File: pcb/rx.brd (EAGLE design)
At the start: 20 x 40 mm, 8 parts, among them IC1 REG1117, IC2 STM32F042K6, J1 USB_A_PTH_MALE

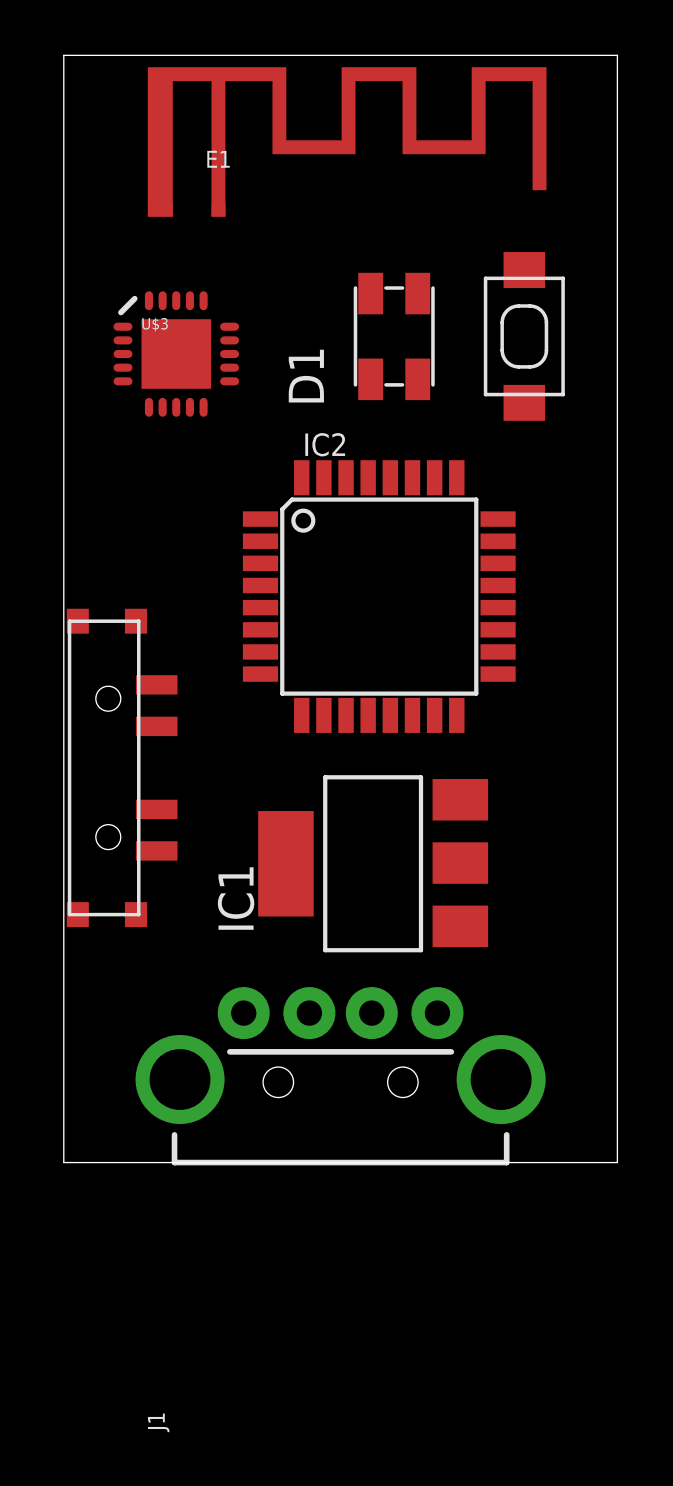
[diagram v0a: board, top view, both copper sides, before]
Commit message: cleanup
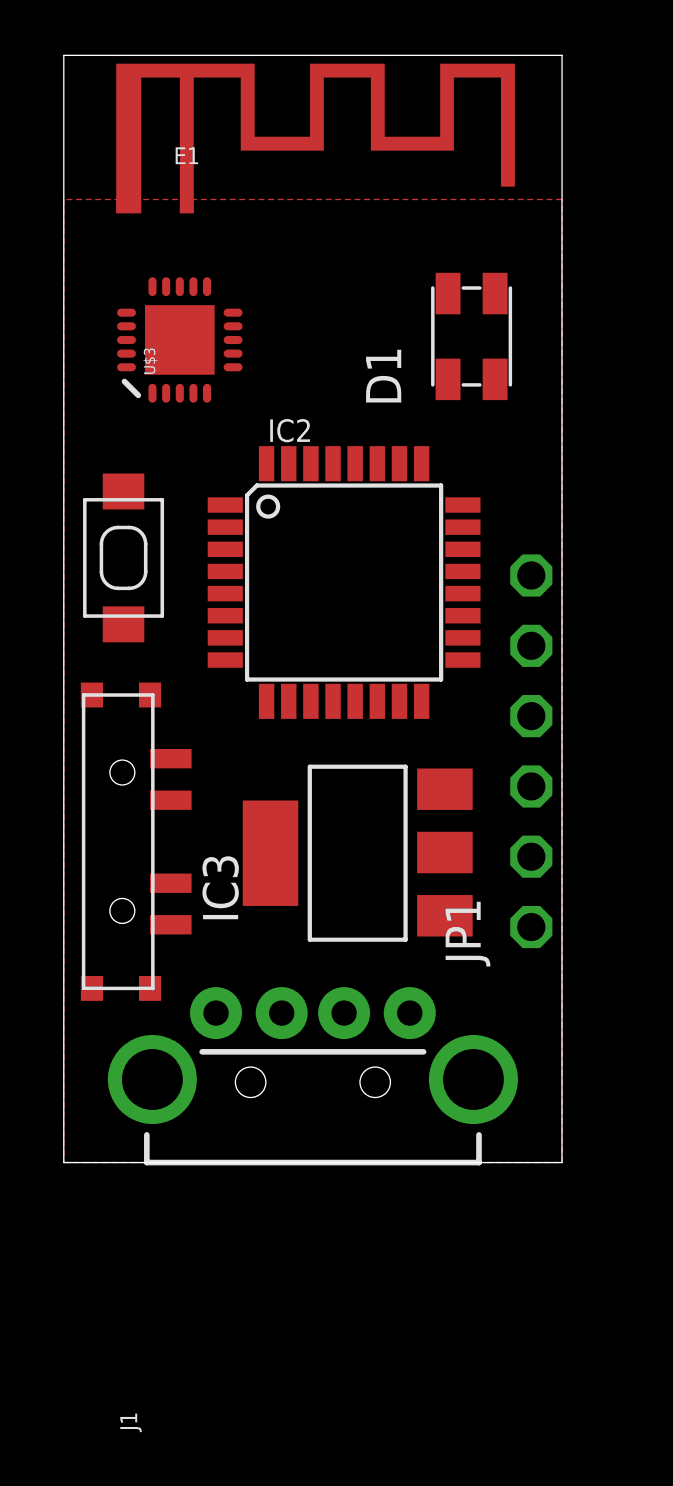
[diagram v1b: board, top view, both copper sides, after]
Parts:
- removed IC1: REG1117, usbclogger:SOT223
- added IC3: REG1117, clock:SOT223
- added JP1: (no value), adafruit:1X06-CLEAN
- moved S1 16.5 mm to (2.16, 21.8)
- moved D1 2.79 mm to (14.7, 29.8)
- moved U$1 2.71 mm to (1.02, 16.9)
- moved IC2 1.37 mm to (10.1, 21.0)
- moved E1 1.15 mm to (4.45, 34.8)
- moved J1 1.00 mm to (9.00, 3.00)
- moved U$3 0.52 mm to (4.19, 29.7), turned to 90 degrees
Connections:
- net GND: now also IC3.1; no longer IC1.1
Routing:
- added copper zone on layer 1, net GND
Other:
- board size 20 x 40 mm -> 18 x 40 mm
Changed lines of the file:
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@@
 <board>
 <plain>
-<wire x1="0" y1="0" x2="20" y2="0" width="0" layer="20"/>
-<wire x1="20" y1="0" x2="20" y2="40" width="0" layer="20"/>
-<wire x1="20" y1="40" x2="0" y2="40" width="0" layer="20"/>
+<wire x1="0" y1="0" x2="18" y2="0" width="0" layer="20"/>
+<wire x1="18" y1="0" x2="18" y2="40" width="0" layer="20"/>
+<wire x1="18" y1="40" x2="0" y2="40" width="0" layer="20"/>
 <wire x1="0" y1="40" x2="0" y2="0" width="0" layer="20"/>
 </plain>
@@
 </autorouter>
 <elements>
-<element name="U$3" library="nRF24L01-Chip-v13" package="QFN20_ALT1" value="NRF24L01ALT1" x="4.064" y="29.21"/>
-<element name="J1" library="SparkFun-Connectors" package="USB-A-H" value="USB_A_PTH_MALE" x="10" y="3" rot="R90">
-<attribute name="PROD_ID" value="CONN-08367" x="10" y="3" size="1.778" layer="27" rot="R90" display="off"/>
-<attribute name="SF_ID" value="PRT-00437" x="10" y="3" size="1.778" layer="27" rot="R90" display="off"/>
+<element name="U$3" library="nRF24L01-Chip-v13" package="QFN20_ALT1" value="NRF24L01ALT1" x="4.191" y="29.718" rot="R90"/>
+<element name="J1" library="SparkFun-Connectors" package="USB-A-H" value="USB_A_PTH_MALE" x="9" y="3" rot="R90">
+<attribute name="PROD_ID" value="CONN-08367" x="9" y="3" size="1.778" layer="27" rot="R90" display="off"/>
+<attribute name="SF_ID" value="PRT-00437" x="9" y="3" size="1.778" layer="27" rot="R90" display="off"/>
 </element>
-<element name="IC2" library="nixx" package="TQFP32-08" value="STM32F042K6" x="11.397" y="20.447"/>
-<element name="E1" library="SparkFun-RF" package="TRACE_ANTENNA_2.4GHZ_15.2MM" value="ANTENNA-GROUNDEDTRACE-15.2MM" x="5.588" y="34.671"/>
-<element name="U$1" library="3pos_slide_switch" package="SW_3POS_FOOT_OFFICIAL" value="SW_3POS_DEVSW_3POS_OFFICIAL" x="0.508" y="19.558" rot="R270"/>
-<element name="IC1" library="usbclogger" package="SOT223" value="REG1117" x="11.176" y="10.795" rot="R90">
-<attribute name="MF" value="" x="-1.397" y="3.302" size="1.778" layer="27" rot="R90" display="off"/>
-<attribute name="MPN" value="REG1117" x="-1.397" y="3.302" size="1.778" layer="27" rot="R90" display="off"/>
-<attribute name="OC_FARNELL" value="1097566" x="-1.397" y="3.302" size="1.778" layer="27" rot="R90" display="off"/>
-<attribute name="OC_NEWARK" value="14P6981" x="-1.397" y="3.302" size="1.778" layer="27" rot="R90" display="off"/>
+<element name="IC2" library="nixx" package="TQFP32-08" value="STM32F042K6" x="10.127" y="20.955"/>
+<element name="E1" library="SparkFun-RF" package="TRACE_ANTENNA_2.4GHZ_15.2MM" value="ANTENNA-GROUNDEDTRACE-15.2MM" x="4.445" y="34.798"/>
+<element name="U$1" library="3pos_slide_switch" package="SW_3POS_FOOT_OFFICIAL" value="SW_3POS_DEVSW_3POS_OFFICIAL" x="1.016" y="16.891" rot="R270"/>
+<element name="S1" library="Adafruit Feather M0 Adalogger" package="KMR2" value="SWITCH-MOMENTARY-2TURTLE" x="2.159" y="21.844" rot="R270"/>
+<element name="D1" library="nixx" package="3528-COMMON-ANODE" value="RGB_LED_CA-150141M173100-R&amp;G&amp;B" x="14.732" y="29.845" rot="R90"/>
+<element name="IC3" library="clock" package="SOT223" value="REG1117" x="10.619" y="11.176" rot="R90">
+<attribute name="MF" value="" x="-1.954" y="3.683" size="1.778" layer="27" rot="R90" display="off"/>
+<attribute name="MPN" value="REG1117" x="-1.954" y="3.683" size="1.778" layer="27" rot="R90" display="off"/>
+<attribute name="OC_FARNELL" value="1097566" x="-1.954" y="3.683" size="1.778" layer="27" rot="R90" display="off"/>
+<attribute name="OC_NEWARK" value="14P6981" x="-1.954" y="3.683" size="1.778" layer="27" rot="R90" display="off"/>
 </element>
-<element name="S1" library="Adafruit Feather M0 Adalogger" package="KMR2" value="SWITCH-MOMENTARY-2TURTLE" x="16.637" y="29.845" rot="R270"/>
-<element name="D1" library="nixx" package="3528-COMMON-ANODE" value="RGB_LED_CA-150141M173100-R&amp;G&amp;B" x="11.938" y="29.845" rot="R90"/>
+<element name="JP1" library="adafruit" package="1X06-CLEAN" value="" x="16.891" y="14.859" rot="R90"/>
 </elements>
 <signals>
@@
 <contactref element="U$3" pad="15"/>
 <contactref element="U$3" pad="18"/>
-<wire x1="4.064" y1="31.1354" x2="5.9894" y2="30.1963" width="0" layer="19" extent="1-1"/>
-<wire x1="3.5709" y1="27.2846" x2="5.9894" y2="30.1963" width="0" layer="19" extent="1-1"/>
+<wire x1="2.2656" y1="29.718" x2="3.2047" y2="31.6434" width="0" layer="19" extent="1-1"/>
+<wire x1="6.1164" y1="29.2249" x2="3.2047" y2="31.6434" width="0" layer="19" extent="1-1"/>
 </signal>
 <signal name="VDD_PA">
@@
 <contactref element="U$3" pad="17"/>
 <contactref element="U$3" pad="20"/>
-<wire x1="3.0777" y1="31.1354" x2="4.5571" y2="31.1354" width="0" layer="19" extent="1-1"/>
-<wire x1="4.064" y1="29.21" x2="4.5571" y2="31.1354" width="0" layer="19" extent="1-1"/>
-<wire x1="4.064" y1="27.2846" x2="4.064" y2="29.21" width="0" layer="19" extent="1-1"/>
-<wire x1="5.9894" y1="29.7031" x2="4.064" y2="29.21" width="0" layer="19" extent="1-1"/>
+<wire x1="4.191" y1="29.718" x2="3.6979" y2="31.6434" width="0" layer="19" extent="1-1"/>
+<wire x1="6.1164" y1="29.718" x2="4.191" y2="29.718" width="0" layer="19" extent="1-1"/>
+<wire x1="2.2656" y1="30.2111" x2="4.191" y2="29.718" width="0" layer="19" extent="1-1"/>
+<wire x1="2.2656" y1="28.7317" x2="2.2656" y2="30.2111" width="0" layer="19" extent="1-1"/>
 </signal>
 <signal name="VBUS">
@@
 <signal name="GND">
 <contactref element="J1" pad="GND"/>
-<contactref element="IC1" pad="1"/>
-<wire x1="6.5" y1="5.4" x2="14.3256" y2="8.5344" width="0" layer="19" extent="1-1"/>
+<polygon width="0.1524" layer="1" isolate="0.254">
+<vertex x="0" y="34.793"/>
+<vertex x="0" y="0"/>
+<vertex x="18" y="0"/>
+<vertex x="18" y="34.793"/>
+</polygon>
+<contactref element="IC3" pad="1"/>
 </signal>
 </signals>

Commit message: dt rx done
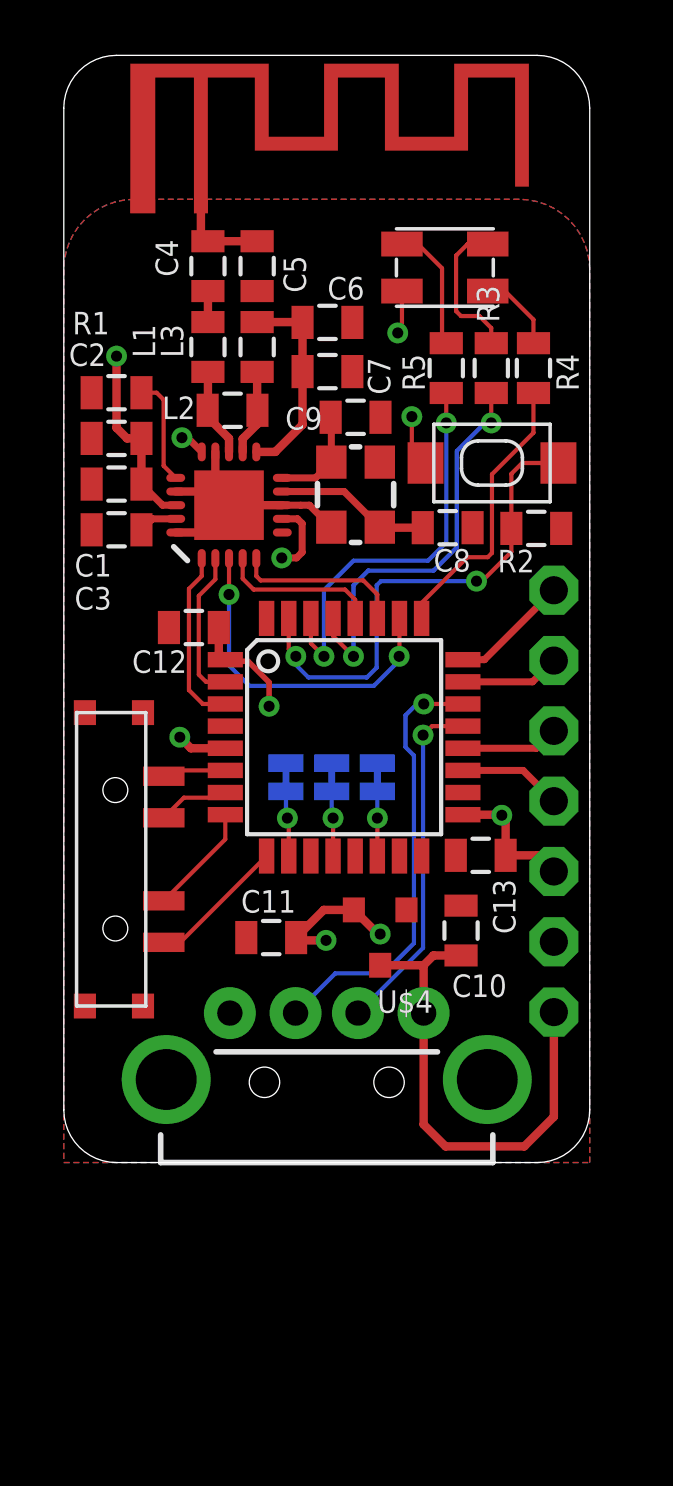
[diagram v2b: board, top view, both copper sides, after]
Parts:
- removed IC3: REG1117, clock:SOT223
- removed JP1: (no value), adafruit:1X06-CLEAN
- added C1, C12, C13, C3: 100nF, clock:0805
- added C10, C11: 1uF, clock:0805
- added C2, C6: 2.2nF, clock:0805
- added C4: 1.5pF, clock:0805
- added C5: 1pF, clock:0805
- added C7: 4.7pF, clock:0805
- added C8, C9: 22pF, clock:0805
- added JP2: (no value), adafruit_changed:1X08-CLEANBIG
- added L1: 3.9nH, basicBoard:0805
- added L2: 8.2nH, basicBoard:0805
- added L3: 2.7nH, basicBoard:0805
- added R1, R2, R3, R4, R5: 22K, joyAnalog:0805
- added SJ1, SJ2, SJ3: JUMPER-SMT_2_NC_TRACE_NO-SILK, SparkFun-Jumpers:SMT-JUMPER_2_NC_TRACE_NO-SILK
- added U$4: XC6206_DEV, 3pos_slide_switch:SOT23R_INFINEON
- added Y1: CRYSTAL-26MHZSMD-3.2X2.5, SparkFun-Clocks:CRYSTAL-SMD-3.2X2.5MM
- moved S1 13.7 mm to (15.5, 25.3), turned to 0 degrees
- moved U$3 6.23 mm to (5.97, 23.7)
- moved IC2 5.59 mm to (10.1, 15.4)
- moved D1 2.67 mm to (13.8, 32.3), turned to 180 degrees
- moved U$1 0.68 mm to (0.76, 16.3)
- moved E1 0.51 mm to (4.95, 34.8)
- moved J1 0.50 mm to (9.50, 3.00)
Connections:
- removed net DVDD: U$3.19
- removed net VBUS: J1.VBUS
- removed net VDD: U$3.15, U$3.18, U$3.7
- removed net VDD_PA: U$3.11
- removed net VSS: U$3.0, U$3.14, U$3.17, U$3.20, U$3.8
- new net +3V3: C1.1, C11.1, C12.1, C13.1, C2.1, D1.1, IC2.1, IC2.17, IC2.5, JP2.5, S1.3, SJ1.1, SJ2.1, SJ3.1, U$3.15, U$3.18, U$3.7, U$4.2
- new net +5V: C10.1, J1.VBUS, JP2.7, U$4.3
- new net N$1: C3.1, U$3.19
- new net N$10: IC2.6, U$1.P$3
- new net N$11: IC2.31, R2.1, S1.1
- new net N$12: IC2.21, J1.D-
- new net N$13: IC2.22, J1.D+
- new net N$14: IC2.28, U$3.4
- new net N$15: IC2.27, U$3.5
- new net N$16: IC2.26, U$3.3
- new net N$17: D1.4, R3.1
- new net N$18: D1.3, R4.1
- new net N$19: D1.2, R5.1
- new net N$2: R1.1, U$3.16
- new net N$20: IC2.2, U$3.2
- new net N$21: IC2.3, U$3.1
- new net N$22: IC2.24, JP2.1
- new net N$23: IC2.23, JP2.2
- new net N$24: IC2.20, JP2.3
- new net N$25: IC2.19, JP2.4
- new net N$26: IC2.7, U$1.P$6
- new net N$27: IC2.8, U$1.P$7
- new net N$28: IC2.9, U$1.P$8
- new net N$29: IC2.25, R4.2
- new net N$3: L1.1, L2.1, U$3.13
- new net N$30: IC2.29, R3.2
- new net N$31: IC2.30, R5.2
- new net N$32: IC2.10, SJ3.2
- new net N$33: IC2.12, SJ2.2
- new net N$34: IC2.14, SJ1.2
- new net N$4: C4.1, L1.2
- new net N$5: C4.2, C5.1, E1.ANT
- new net N$6: L2.2, L3.1, U$3.12
- new net N$7: C8.1, U$3.9, Y1.1
- new net N$8: C6.1, C7.1, L3.2, U$3.11
- new net N$9: C9.1, U$3.10, Y1.3
- net GND: now also C1.2, C10.2, C11.2, C12.2, C13.2, C2.2, C3.2, C5.2, C6.2, C7.2, C8.2, C9.2, E1.GND, IC2.16, IC2.32, J1.SHLD1, J1.SHLD2, JP2.6, R1.2, R2.2, U$1.P$1, U$1.P$2, U$1.P$4, U$1.P$5, U$3.0, U$3.14, U$3.17, U$3.20, U$3.8, U$4.1, Y1.2, Y1.4; no longer IC3.1
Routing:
- net +3V3: track 0.00 -> 29.6 mm, vias 0 -> 10
- net +5V: track 0.00 -> 18.1 mm
- net N$11: track 0.00 -> 18.1 mm, vias 0 -> 2
- net N$13: track 0.00 -> 15.9 mm, vias 0 -> 1
- net N$30: track 0.00 -> 14.8 mm, vias 0 -> 2
- net N$31: track 0.00 -> 14.5 mm, vias 0 -> 2
- net N$12: track 0.00 -> 12.6 mm, vias 0 -> 1
- net N$16: track 0.00 -> 12.2 mm, vias 0 -> 2
- net GND: track 0.00 -> 10.8 mm
- net N$29: track 0.00 -> 10.2 mm
- net N$8: track 0.00 -> 7.42 mm
- net N$21: track 0.00 -> 6.47 mm
- net N$15: track 0.00 -> 6.15 mm
- net N$14: track 0.00 -> 5.78 mm
- net N$7: track 0.00 -> 5.64 mm
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- added copper zone on layer 16, net +3V3
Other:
- board size 18 x 40 mm -> 19 x 40 mm
- board text added: "0"
- board text added: "1"
- board text added: "2"
- board text added: "3V3"
- board text added: "5V"
- board text added: "CLK"
- board text added: "CSTM"
- board text added: "DIO"
- board text added: "GND"
- board text added: "IRQ"
- board text added: "LOCK"
- board text added: "MINI"
- board text added: "TX"
- board text added: "dayTripper RX dekuNukem 2018"
- board text added: "git.io/daytripper"

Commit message: cleanup
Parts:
- C10, C11: value 1uF -> 4.7uF
- R2: value 22K -> 10K
- R3: value 22K -> 4.7K
- R4, R5: value 22K -> 2.2K
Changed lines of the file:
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@@
 <attribute name="VALUE" x="13.335" y="11.303" size="1.27" layer="27" rot="R180"/>
 </element>
-<element name="C10" library="clock" package="0805" value="1uF" x="14.351" y="8.382" smashed="yes" rot="R90">
+<element name="C10" library="clock" package="0805" value="4.7uF" x="14.351" y="8.382" smashed="yes" rot="R90">
 <attribute name="NAME" x="16.002" y="6.7945" size="0.8128" layer="25" rot="R180"/>
 </element>
-<element name="C11" library="clock" package="0805" value="1uF" x="7.493" y="8.128" smashed="yes" rot="R180">
+<element name="C11" library="clock" package="0805" value="4.7uF" x="7.493" y="8.128" smashed="yes" rot="R180">
 <attribute name="NAME" x="8.382" y="9.8425" size="0.8128" layer="25" rot="R180"/>
 </element>
@@
 <attribute name="VALUE" x="12.065" y="24.13" size="0.6096" layer="27" font="vector" ratio="20" rot="R90" align="top-center"/>
 </element>
-<element name="R2" library="joyAnalog" package="0805" value="22K" x="17.0688" y="22.9108" smashed="yes">
+<element name="R2" library="joyAnalog" package="0805" value="10K" x="17.0688" y="22.9108" smashed="yes">
 <attribute name="NAME" x="15.6718" y="21.3233" size="0.8128" layer="25"/>
 <attribute name="VALUE" x="16.0528" y="21.5138" size="0.4064" layer="27"/>
@@
 <attribute name="NAME" x="15.5067" y="10.2362" size="0.8128" layer="25" rot="R270"/>
 </element>
-<element name="R3" library="joyAnalog" package="0805" value="22K" x="15.4432" y="28.702" smashed="yes" rot="R270">
+<element name="R3" library="joyAnalog" package="0805" value="4.7K" x="15.4432" y="28.702" smashed="yes" rot="R270">
 <attribute name="NAME" x="15.7353" y="30.353" size="0.8128" layer="25" rot="R90"/>
 <attribute name="VALUE" x="14.0462" y="29.718" size="0.4064" layer="27" rot="R270"/>
 <attribute name="VALUE" x="14.0462" y="29.718" size="0.4064" layer="27" rot="R270"/>
 </element>
-<element name="R4" library="joyAnalog" package="0805" value="22K" x="16.9672" y="28.702" smashed="yes" rot="R270">
+<element name="R4" library="joyAnalog" package="0805" value="2.2K" x="16.9672" y="28.702" smashed="yes" rot="R270">
 <attribute name="NAME" x="17.7927" y="29.21" size="0.8128" layer="25" rot="R270"/>
 <attribute name="VALUE" x="15.5702" y="29.718" size="0.4064" layer="27" rot="R270"/>
 <attribute name="VALUE" x="15.5702" y="29.718" size="0.4064" layer="27" rot="R270"/>
 </element>
-<element name="R5" library="joyAnalog" package="0805" value="22K" x="13.8176" y="28.702" smashed="yes" rot="R270">
+<element name="R5" library="joyAnalog" package="0805" value="2.2K" x="13.8176" y="28.702" smashed="yes" rot="R270">
 <attribute name="NAME" x="12.2301" y="29.21" size="0.8128" layer="25" rot="R270"/>
 <attribute name="VALUE" x="12.4206" y="29.718" size="0.4064" layer="27" rot="R270"/>
